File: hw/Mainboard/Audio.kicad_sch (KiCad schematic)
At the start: 11 parts, among them J1 SJ-43504-SMT-TR, J8 SPEAKER, Q2 MMBT3904

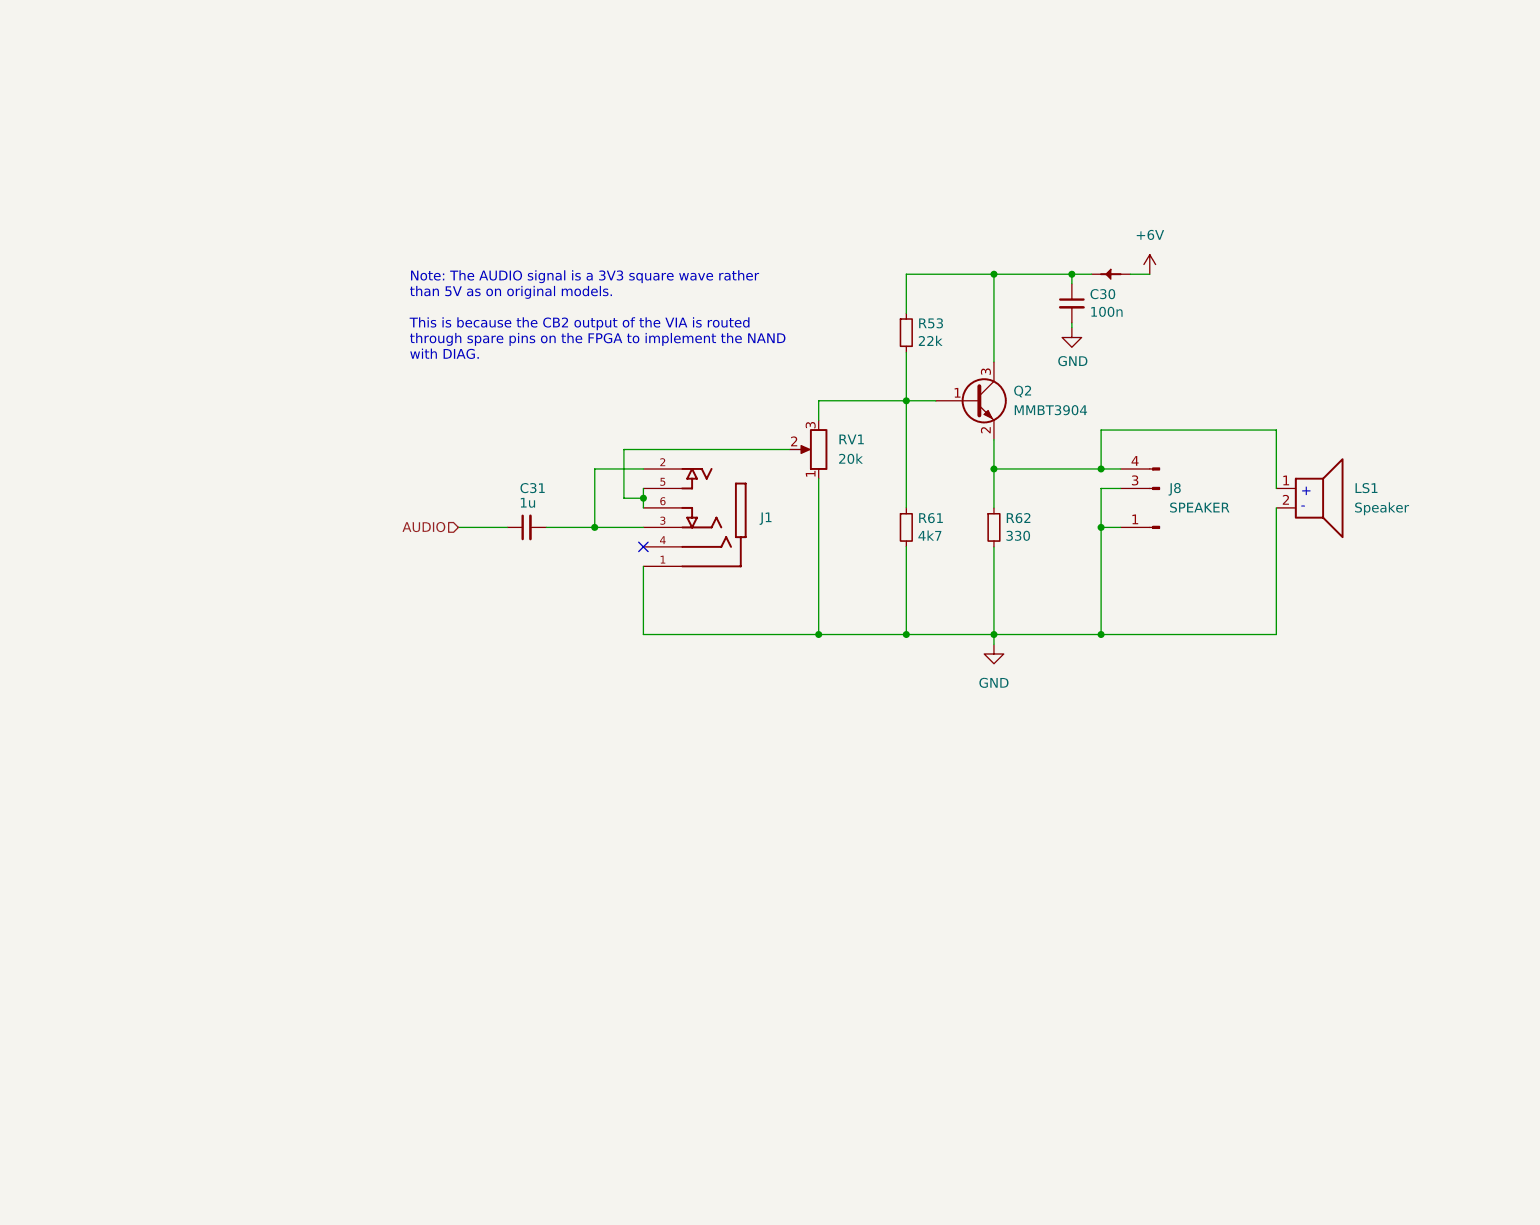
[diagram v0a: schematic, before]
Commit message: hw: autoroute
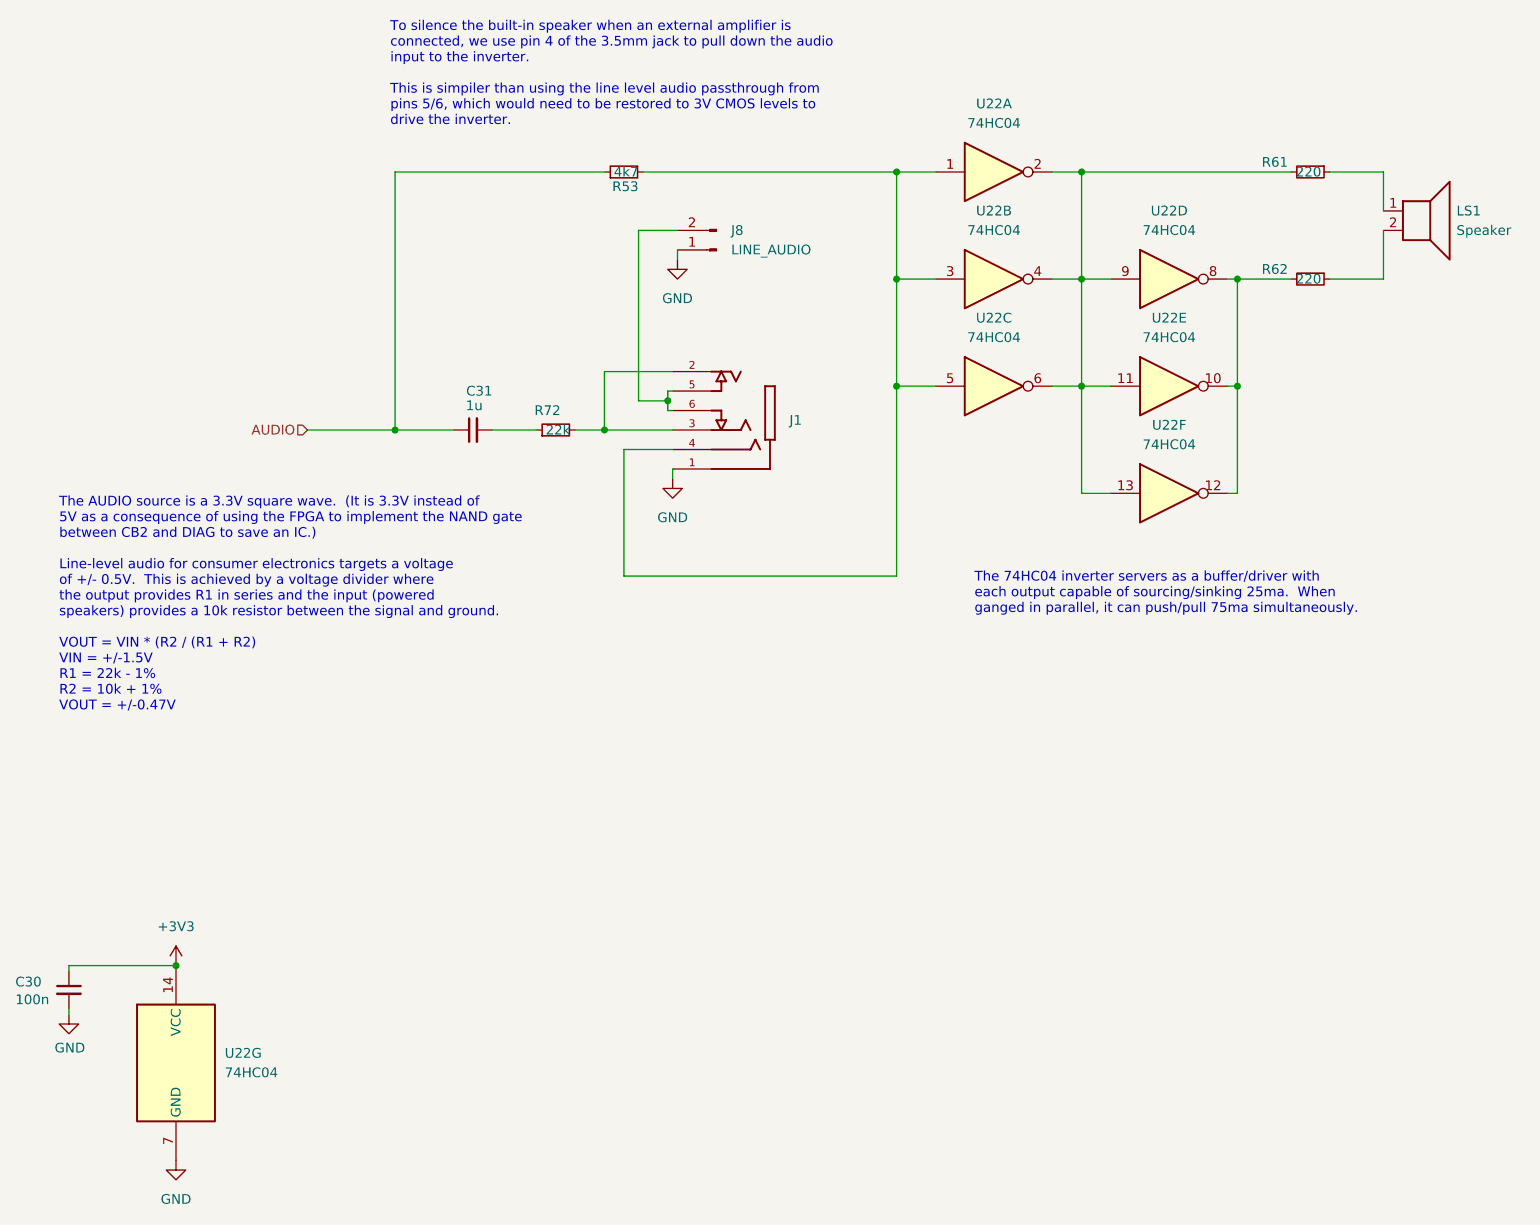
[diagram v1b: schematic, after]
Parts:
- removed J8: SPEAKER, PET:PET_SPEAKER, symbol PET:PET_SPEAKER_01x04_Male
- removed PT26: PowerTie_2, PET:NetTie-2_SMD_Pad_1.6_to_0.4mm, symbol PET:PowerTie_2
- removed Q2: MMBT3904, Package_TO_SOT_SMD:SOT-23, symbol Transistor_BJT:MMBT3904
- removed RV1: 20k, Potentiometer_SMD:Potentiometer_Bourns_TC33X_Vertical, symbol Device:R_Potentiometer
- added J8: LINE_AUDIO, Connector_PinHeader_2.54mm:PinHeader_1x02_P2.54mm_Vertical, symbol Connector:Conn_01x02_Male
- added R72: 22k, Resistor_SMD:R_0402_1005Metric, symbol Device:R_Small
- added U22: 74HC04, symbol 74xx:74HC04
- LS1: footprint SnapEDA:XDCR_AT-1224-TWT-5V-2-R -> SamacSys_Parts:AT1220TT9R; MOUSER 665-AT1224TWT5V2R -> 665-AT1220TT9R; MPN AT-1224-TWT-5V-2-R -> (none)
- R53: value 22k -> 4k7; LCSC C25768 -> C25900
- R61: value 4k7 -> 220; footprint Resistor_SMD:R_0402_1005Metric -> Resistor_SMD:R_0603_1608Metric; LCSC C25900 -> C22962
- R62: value 330 -> 220; footprint Resistor_SMD:R_0805_2012Metric -> Resistor_SMD:R_0603_1608Metric; LCSC C17630 -> C22962
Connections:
- net AUDIO: now also R53.1
- net GND: now also J8.1 (Pin_1), U22.7 (GND); no longer LS1.2, R61.2, R62.2
- net +3V3: now reaches C30.1
- net +3V3: now also U22.14 (VCC); no longer R53.1
- net at LS1.1: now also R61.1; no longer R62.1
- net at R53.2: now also J1.4, U22.1, U22.3, U22.5; no longer R61.1
- net at J1.2, J1.3: now also R72.2; no longer C31.2
- net at J1.5, J1.6: now also J8.2 (Pin_2)
- new net: C31.2, R72.1
- new net: R61.2, U22.11, U22.13, U22.2, U22.4, U22.6, U22.9
- new net: LS1.2, R62.1
- new net: R62.2, U22.10, U22.12, U22.8
- no-connect marks 1 -> 0
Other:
- note added: "The 74HC04 inverter servers as a buffer/driver with each output capable of sourcing/sinking 25ma. When ganged in parallel, it can push/pull 75ma simultaneously."
- note added: "The AUDIO source is a 3.3V square wave. (It is 3.3V instead of 5V as a consequence of using the FPGA to implement the NAND gate between CB2 and DIAG to save an IC.) Line-level audio for consumer electronics targets a voltage of +/- 0.5V. This is achieved by a voltage divider where the output provides R1 in series and the input (powered speakers) provides a 10k resistor between the signal and grou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"
- note added: "To silence the built-in speaker when an external amplifier is connected, we use pin 4 of the 3.5mm jack to pull down the audio input to the inverter. This is simpiler than using the line level audio passthrough from pins 5/6, which would need to be restored to 3V CMOS levels to drive the inverter."
- note removed: "+"
- note removed: "-"
- note removed: "Note: The AUDIO signal is a 3V3 square wave rather than 5V as on original models. This is because the CB2 output of the VIA is routed through spare pins on the FPGA to implement the NAND with DIAG."
- moved on the sheet: C30, C31, J1

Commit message: hw: wip
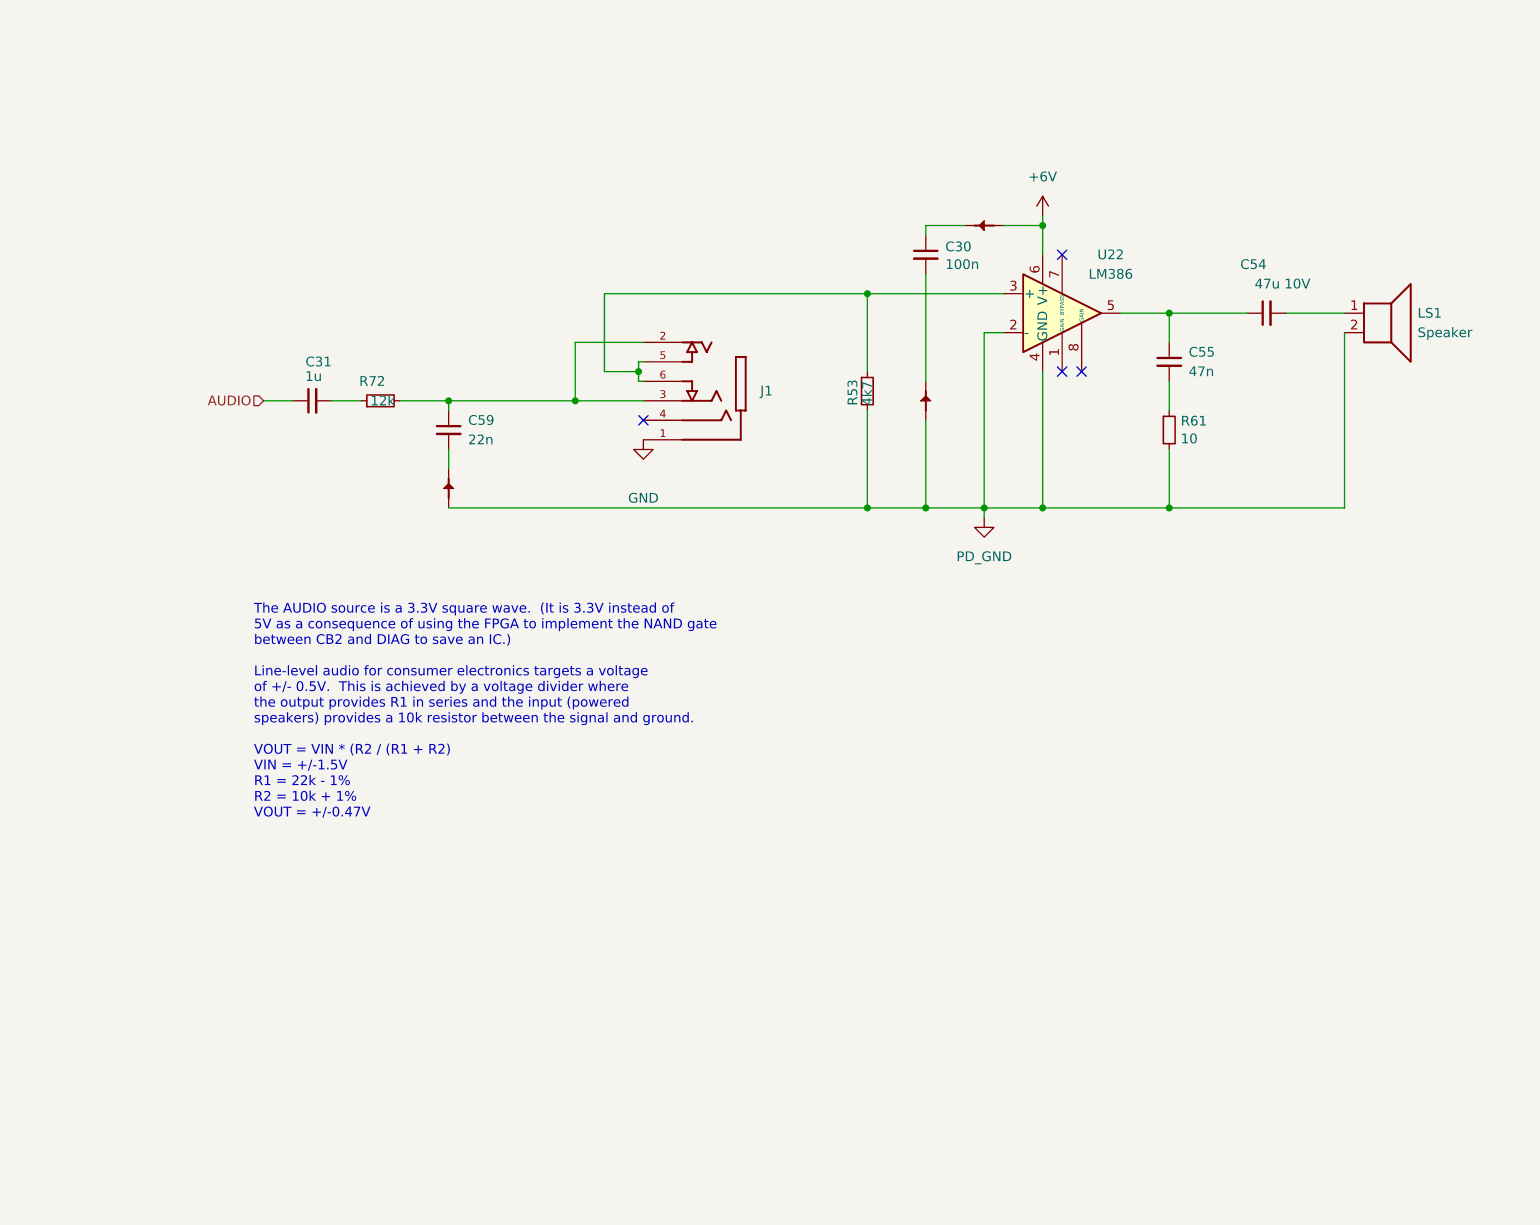
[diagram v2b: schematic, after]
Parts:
- removed J8: LINE_AUDIO, Connector_PinHeader_2.54mm:PinHeader_1x02_P2.54mm_Vertical, symbol Connector:Conn_01x02_Male
- removed R62: 220, Resistor_SMD:R_0603_1608Metric, symbol Device:R_Small
- removed U22: 74HC04, symbol 74xx:74HC04
- added C54: 47u 10V, Capacitor_SMD:C_1206_3216Metric, symbol Device:C_Small
- added C55: 47n, Capacitor_SMD:C_0402_1005Metric, symbol Device:C_Small
- added C59: 22n, Capacitor_SMD:C_0402_1005Metric, symbol Device:C_Small
- added PT35, PT36, PT38: PowerTie_2, PET:NetTie-2_SMD_Pad_1.6_to_0.4mm, symbol PET:PowerTie_2
- added U22: LM386, Package_DIP:DIP-8_W7.62mm, symbol Amplifier_Audio:LM386
- R53: footprint Resistor_SMD:R_0402_1005Metric -> Resistor_SMD:R_0805_2012Metric_Pad1.20x1.40mm_HandSolder; LCSC C25900 -> C17673
- R61: value 220 -> 10; footprint Resistor_SMD:R_0603_1608Metric -> Resistor_SMD:R_0805_2012Metric_Pad1.20x1.40mm_HandSolder; LCSC C22962 -> C17415
- R72: value 22k -> 12k; footprint Resistor_SMD:R_0402_1005Metric -> Resistor_SMD:R_0805_2012Metric_Pad1.20x1.40mm_HandSolder; LCSC C25768 -> C17444
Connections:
- net AUDIO: no longer R53.1
- net GND: no longer C30.2
- net at J1.2, J1.3, R72.2: now also C59.1
- net at R61.1: now also C55.2; no longer LS1.1
- net PD_GND: now reaches R61.2
- net PD_GND: now also LS1.2, R53.2, PT36.1, PT38.1, U22.2 (-), U22.4 (GND)
- net at J1.4: no longer R53.2
- net at J1.5, J1.6: now also R53.1, U22.3 (+)
- net +3V3: no longer names the net of C30.1
- net +3V3: now also PT35.2
- new net: C30.2, PT36.2
- new net: C59.2, PT38.2
- new net: C54.2, LS1.1
- new net: C54.1, C55.1, U22.5
- new net +6V: PT35.1, U22.6 (V+)
- no-connect marks 0 -> 4
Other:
- note removed: "The 74HC04 inverter servers as a buffer/driver with each output capable of sourcing/sinking 25ma. When ganged in parallel, it can push/pull 75ma simultaneously."
- note removed: "To silence the built-in speaker when an external amplifier is connected, we use pin 4 of the 3.5mm jack to pull down the audio input to the inverter. This is simpiler than using the line level audio passthrough from pins 5/6, which would need to be restored to 3V CMOS levels to drive the inverter."
- moved on the sheet: C30, C31, J1, LS1, R72
